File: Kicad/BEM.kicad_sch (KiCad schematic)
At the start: 18 parts, among them J2 SD_Card_Device, U2 ACS712xLCTR-30A, U3 ACS712xLCTR-30A, U4 ACS712xLCTR-30A, U5 ACS712xLCTR-30A

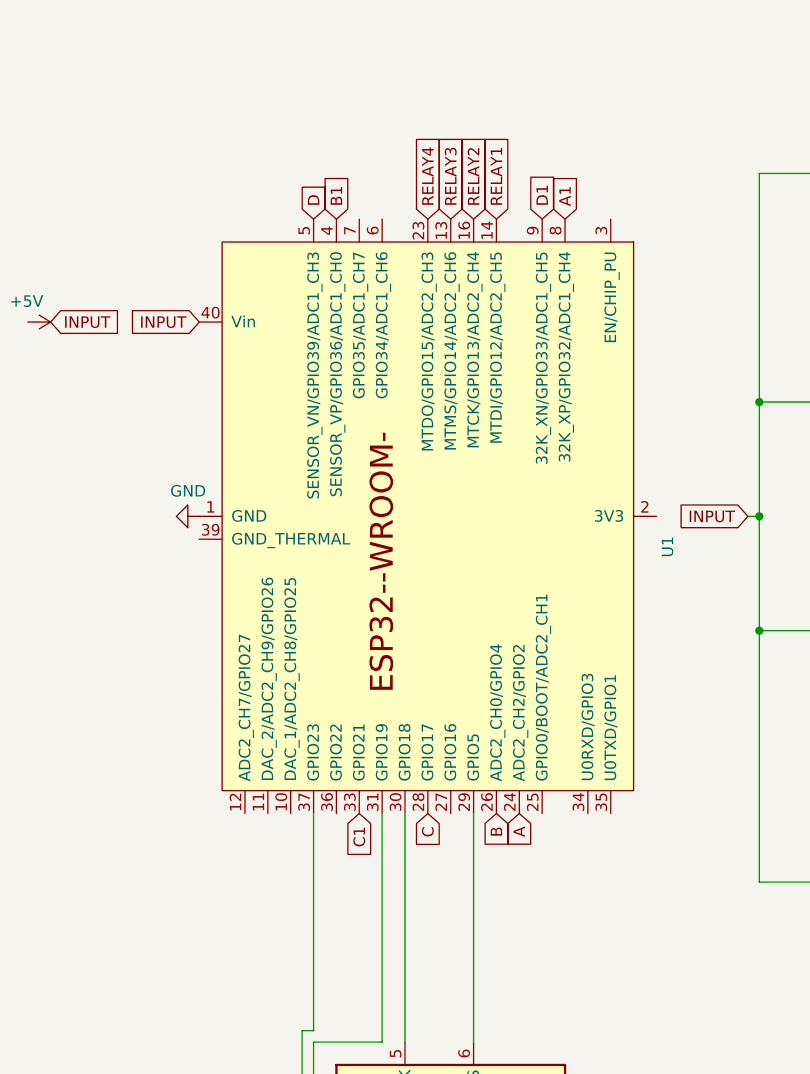
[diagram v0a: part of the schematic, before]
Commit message: Schematic
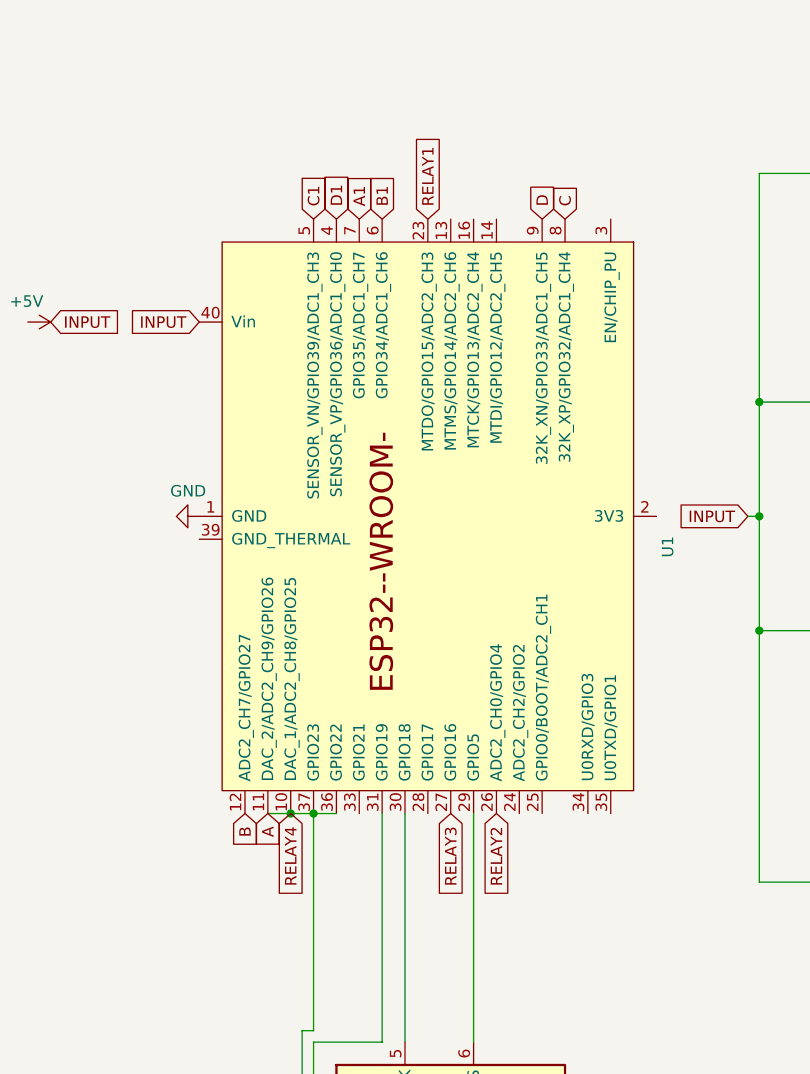
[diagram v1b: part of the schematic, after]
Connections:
- net A: now also J2.3 (MOSI), K4.1, U1.10 (DAC_1/ADC2_CH8/GPIO25), U1.11 (DAC_2/ADC2_CH9/GPIO26), U1.36 (GPIO22), U1.37 (GPIO23); no longer U1.24 (ADC2_CH2/GPIO2)
- net A1: now also U1.7 (GPIO35/ADC1_CH7); no longer U1.8 (32K_XP/GPIO32/ADC1_CH4)
- net B: now also U1.12 (ADC2_CH7/GPIO27); no longer U1.26 (ADC2_CH0/GPIO4)
- net B1: now also U1.6 (GPIO34/ADC1_CH6); no longer U1.4 (SENSOR_VP/GPIO36/ADC1_CH0)
- net C: now also U1.8 (32K_XP/GPIO32/ADC1_CH4); no longer U1.28 (GPIO17)
- net C1: now also U1.5 (SENSOR_VN/GPIO39/ADC1_CH3); no longer U1.33 (GPIO21)
- net D: now also U1.9 (32K_XN/GPIO33/ADC1_CH5); no longer U1.5 (SENSOR_VN/GPIO39/ADC1_CH3)
- net D1: now also U1.4 (SENSOR_VP/GPIO36/ADC1_CH0); no longer U1.9 (32K_XN/GPIO33/ADC1_CH5)
- net RELAY1: now also U1.23 (MTDO/GPIO15/ADC2_CH3); no longer U1.14 (MTDI/GPIO12/ADC2_CH5)
- net RELAY2: now also U1.26 (ADC2_CH0/GPIO4); no longer U1.16 (MTCK/GPIO13/ADC2_CH4)
- net RELAY3: now also U1.27 (GPIO16); no longer U1.13 (MTMS/GPIO14/ADC2_CH6)
- removed net RELAY4: K4.1, U1.23 (MTDO/GPIO15/ADC2_CH3)
